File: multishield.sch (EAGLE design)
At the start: 24 parts, among them CN1 3P-2.54-90D, J1 7p-2.54-90d, J2 2x16p-2.54, J3 7p-2.54-90d, J4 2x6p-2.54, J5 7p-2.54-90d, J6 7p-2.54-90d, K2 TS-1101F, M1 ARDUINO_R3_ICSP, SW1 SK-12D01, U1 AD595AQ-DIP14, U2 ATMEGA328P_PDIP, Y1 16MHZ

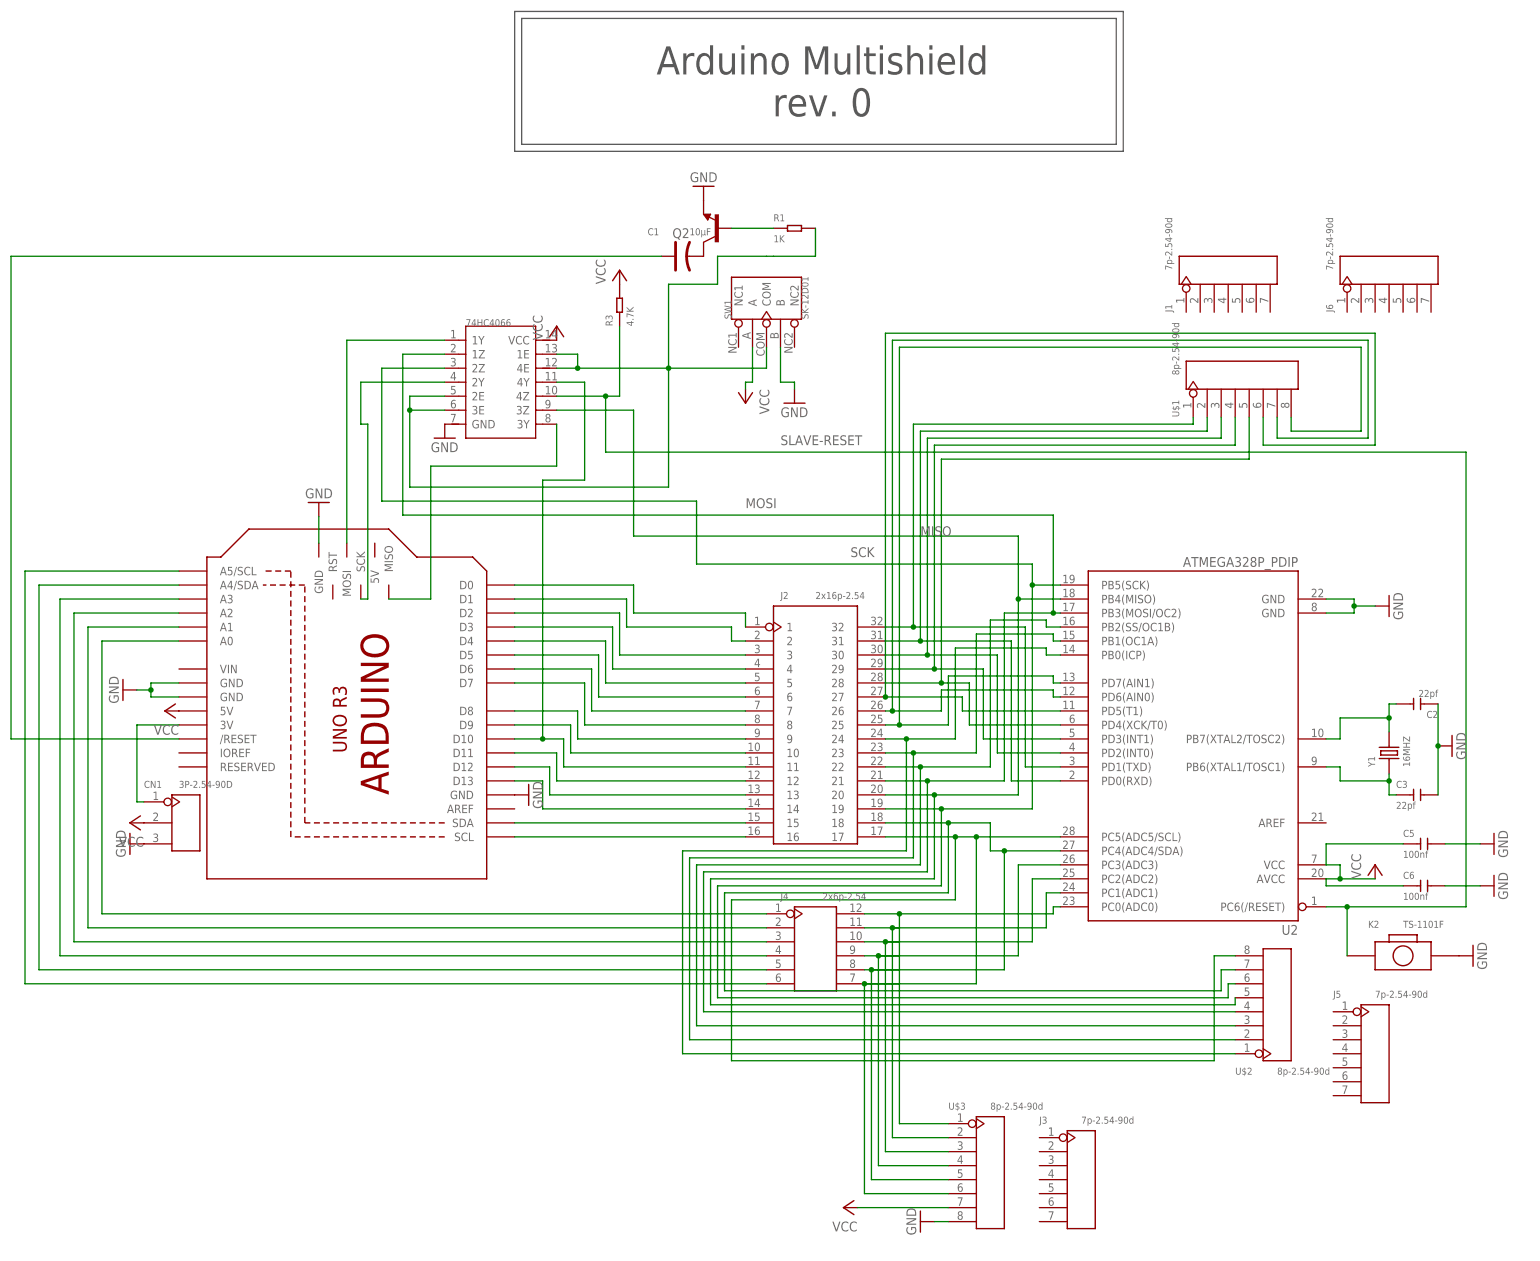
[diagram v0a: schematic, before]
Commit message: 7pin angled headers instead
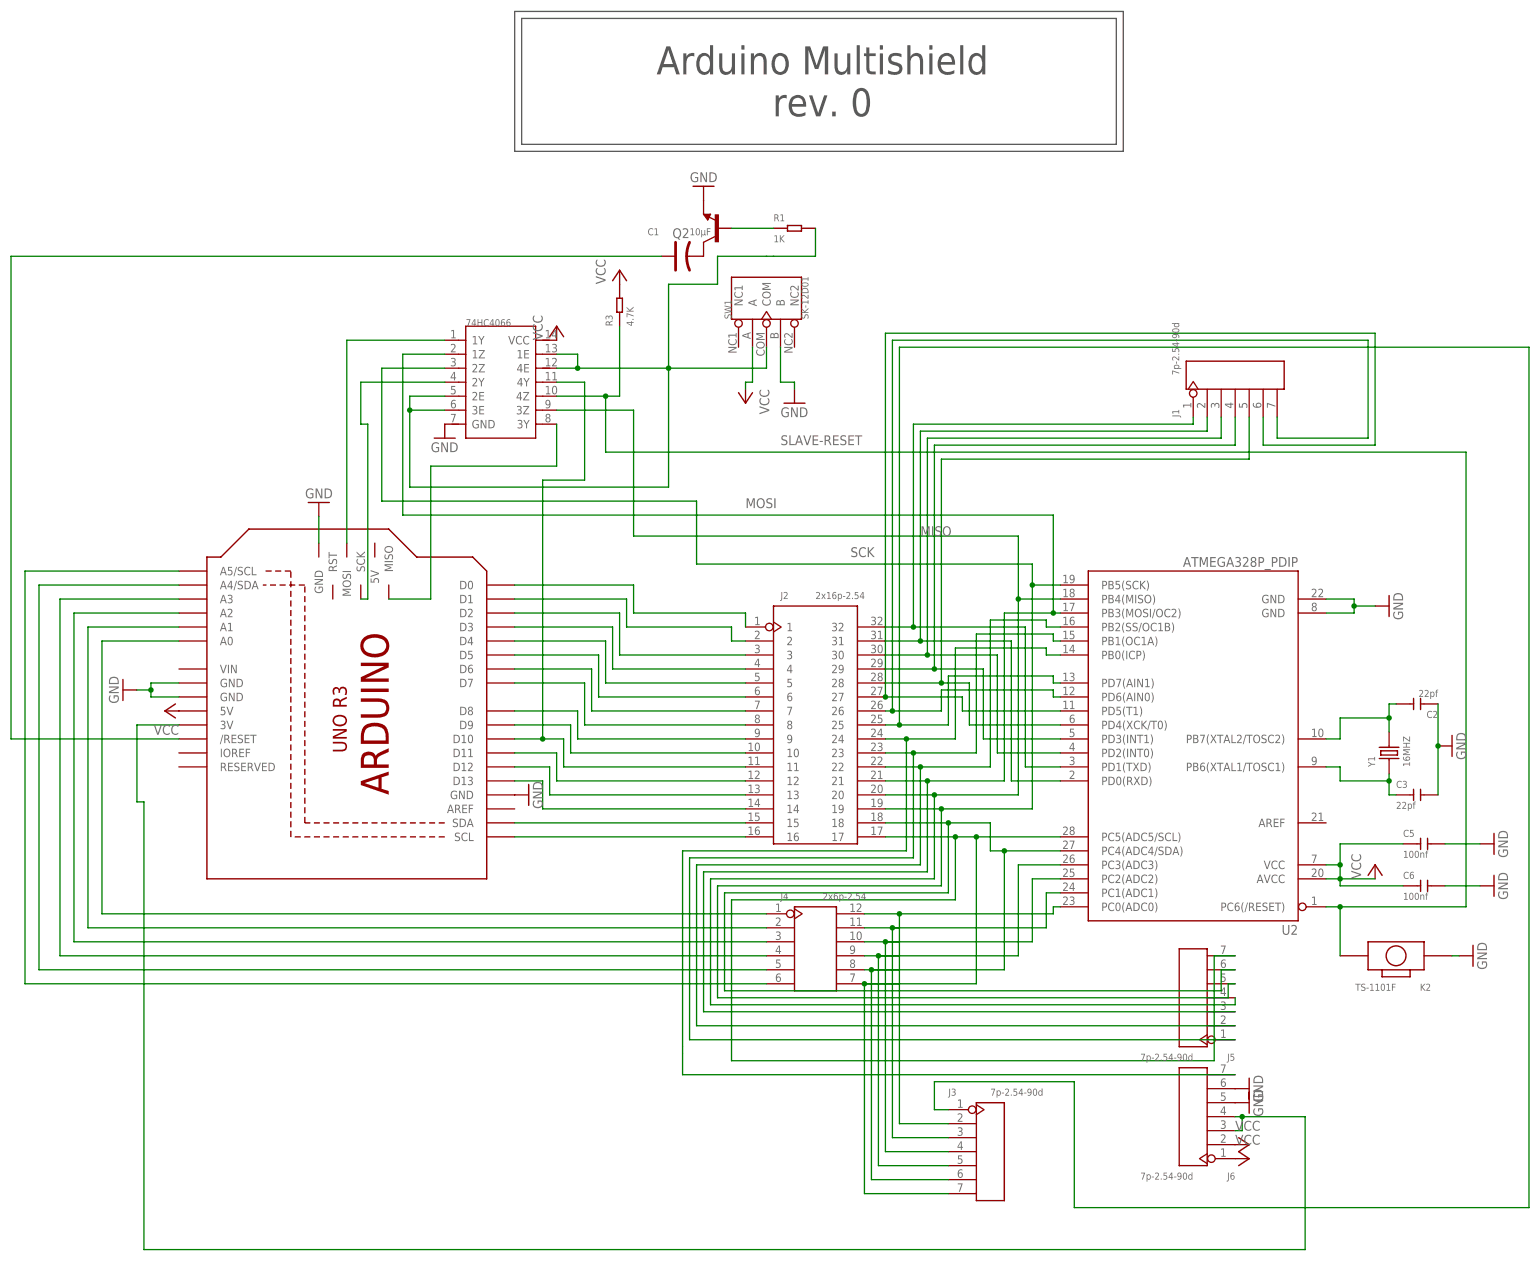
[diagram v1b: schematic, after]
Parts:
- removed CN1: 3P-2.54-90D, Seeed-OPL-Connector:DIP-BLACK-FEMALE-HEADER(3P-2.54-90D)
- removed U$1, U$2, U$3: 8p-2.54-90d, Seeed-OPL-Connector:DIP-BLACK-FEMALE-HEADER-R/A(8P-2.54-90D)
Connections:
- net GND: now also J6.5, J6.6, K2.1; no longer CN1.P$3, K2.2, U$3.8
- net MISO: now also J5.4; no longer U$2.5
- net MOSI: now also J5.3; no longer U$2.4
- net N$25: now also J1.1; no longer U$1.1
- net N$26: now also J1.2; no longer U$1.2
- net N$27: now also J1.3; no longer U$1.3
- net N$28: now also J1.4; no longer U$1.4
- net N$29: now also J1.5; no longer U$1.5
- net N$30: now also J1.6; no longer U$1.6
- net N$32: now also J3.1; no longer U$1.8
- net N$33: now also J6.7; no longer U$2.1
- net N$34: now also J5.1; no longer U$2.2
- net N$35: now also J5.2; no longer U$2.3
- net N$41: now also J1.7; no longer U$1.7
- net N$45: now also J3.2; no longer U$3.1
- net N$46: now also J3.3; no longer U$3.2
- net N$47: now also J3.4; no longer U$3.3
- net N$48: now also J3.5; no longer U$3.4
- net N$49: now also J3.6, J5.6; no longer U$2.7, U$3.5
- net N$50: now also J3.7, J5.7; no longer U$2.8, U$3.6
- net N$54: now also J6.3, J6.4; no longer CN1.P$1
- net SCK: now also J5.5; no longer U$2.6
- net SLAVE-RESET: now also K2.2; no longer K2.1
- net VCC: now also J6.1, J6.2; no longer CN1.P$2, U$3.7
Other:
- moved on the sheet: J1, J3, J5, J6, K2
